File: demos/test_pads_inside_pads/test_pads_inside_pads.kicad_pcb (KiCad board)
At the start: 2 copper layers, 4 parts, among them P1 CONN_1, P2 CONN_1, P3 CONN_1, P4 CONN_1

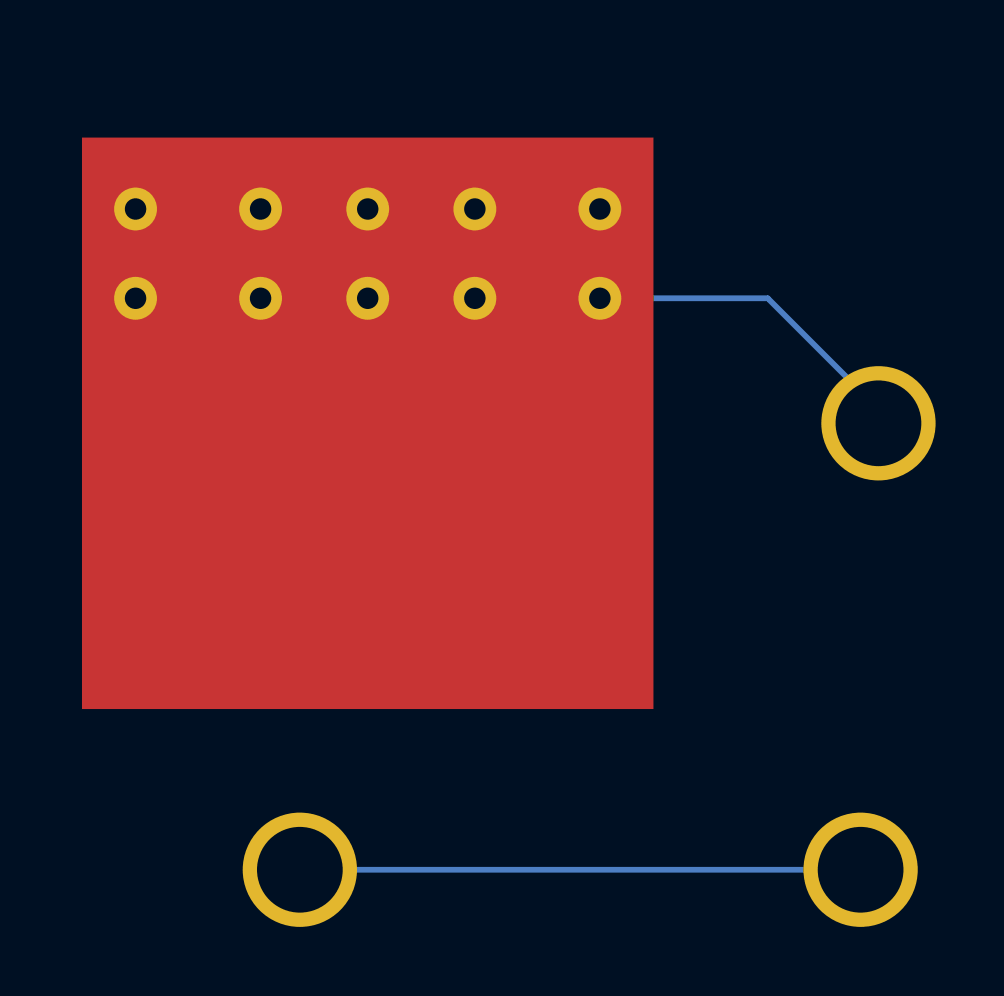
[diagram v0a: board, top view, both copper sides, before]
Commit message: Imported Upstream version 4.0.0~rc1
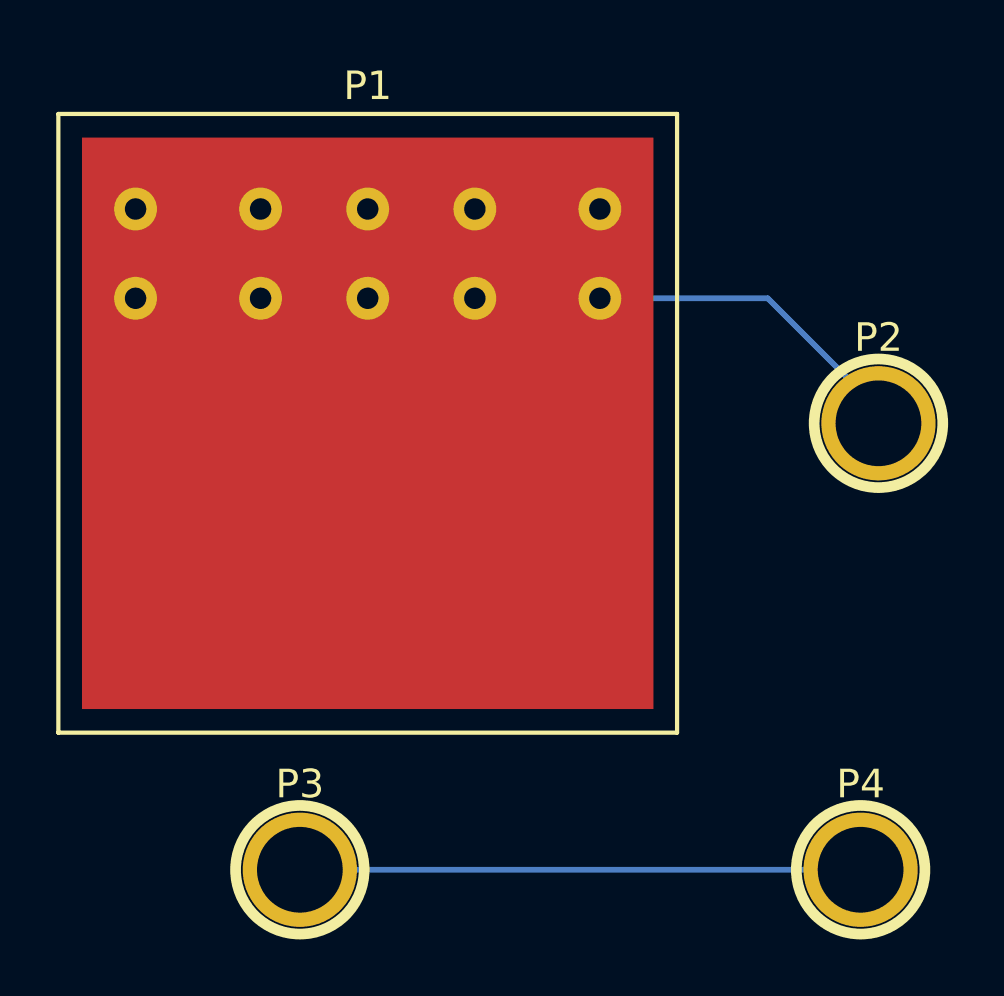
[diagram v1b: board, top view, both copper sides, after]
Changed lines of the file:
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@@
-(kicad_pcb (version 3) (host pcbnew "(2013-01-12 BZR 3902)-testing")
+(kicad_pcb (version 4) (host pcbnew "(2015-04-25 BZR 5623)-product")
   (general
     (links 12)
     (no_connects 0)
-    (area 74.91259 30.97059 111.463666 65.151)
+    (area 79.121 35.179 111.052429 65.3542)
     (thickness 1.6002)
     (drawings 0)
@@
   (page A4)
   (layers
-    (15 Dessus signal)
-    (0 Dessous signal)
-    (16 Dessous.Adhes user)
-    (17 Dessus.Adhes user)
-    (18 Dessous.Pate user)
-    (19 Dessus.Pate user)
-    (20 Dessous.SilkS user)
-    (21 Dessus.SilkS user)
-    (22 Dessous.Masque user)
-    (23 Dessus.Masque user)
-    (24 Dessin.User user)
-    (25 Cmts.User user)
-    (26 Eco1.User user)
-    (27 Eco2.User user)
-    (28 Contours.Ci user)
+    (0 Dessus signal)
+    (31 Dessous signal)
+    (32 B.Adhes user)
+    (33 F.Adhes user)
+    (34 B.Paste user)
+    (35 F.Paste user)
+    (36 B.SilkS user)
+    (37 F.SilkS user)
+    (38 B.Mask user)
+    (39 F.Mask user)
+    (40 Dwgs.User user)
+    (41 Cmts.User user)
+    (42 Eco1.User user)
+    (43 Eco2.User user)
+    (44 Edge.Cuts user)
   )
   (setup
@@
     (pad_to_mask_clearance 0.254)
     (aux_axis_origin 0 0)
-    (visible_elements FFFFFFBF)
+    (visible_elements 7FFFFFFF)
     (pcbplotparams
-      (layerselection 3178497)
+      (layerselection 0x00030_80000001)
       (usegerberextensions true)
       (excludeedgelayer true)
-      (linewidth 60)
+      (linewidth 0.150000)
       (plotframeref false)
       (viasonmask false)
@@
       (plotreference true)
       (plotvalue true)
-      (plotothertext true)
       (plotinvisibletext false)
       (padsonsilk false)
@@
     (uvia_dia 0.508)
     (uvia_drill 0.127)
-    (add_net "")
     (add_net /NET1)
     (add_net /NET2)
@@
     (descr "module 1 pin (ou trou mecanique de percage)")
     (tags DEV)
-    (fp_text reference P1 (at 0 -3.048) (layer Dessus.SilkS)
+    (fp_text reference P1 (at 0 -12) (layer F.SilkS)
       (effects (font (size 1.016 1.016) (thickness 0.254)))
     )
-    (fp_text value CONN_1 (at 0 2.794) (layer Dessus.SilkS) hide
+    (fp_text value CONN_1 (at 0 12) (layer F.SilkS) hide
       (effects (font (size 1.016 1.016) (thickness 0.254)))
     )
-    (fp_circle (center 0 0) (end 0 -2.286) (layer Dessus.SilkS) (width 0.381))
-    (pad 1 smd rect (at 0 0) (size 20.32 20.32)
-      (layers Dessus Dessus.Pate Dessus.Masque)
-      (net 2 /NET2)
-    )
-    (pad 1 thru_hole circle (at -8.255 -7.62) (size 1.524 1.524) (drill 0.762)
-      (layers *.Cu *.Mask Dessus.SilkS)
-      (net 2 /NET2)
-    )
-    (pad 1 thru_hole circle (at -3.81 -7.62) (size 1.524 1.524) (drill 0.762)
-      (layers *.Cu *.Mask Dessus.SilkS)
-      (net 2 /NET2)
-    )
-    (pad 1 thru_hole circle (at 0 -7.62) (size 1.524 1.524) (drill 0.762)
-      (layers *.Cu *.Mask Dessus.SilkS)
-      (net 2 /NET2)
-    )
-    (pad 1 thru_hole circle (at 3.81 -7.62) (size 1.524 1.524) (drill 0.762)
-      (layers *.Cu *.Mask Dessus.SilkS)
-      (net 2 /NET2)
-    )
-    (pad 1 thru_hole circle (at 8.255 -7.62) (size 1.524 1.524) (drill 0.762)
-      (layers *.Cu *.Mask Dessus.SilkS)
-      (net 2 /NET2)
-    )
-    (pad 1 thru_hole circle (at 8.255 -4.445) (size 1.524 1.524) (drill 0.762)
-      (layers *.Cu *.Mask Dessus.SilkS)
-      (net 2 /NET2)
-    )
-    (pad 1 thru_hole circle (at 3.81 -4.445) (size 1.524 1.524) (drill 0.762)
-      (layers *.Cu *.Mask Dessus.SilkS)
-      (net 2 /NET2)
-    )
-    (pad 1 thru_hole circle (at 0 -4.445) (size 1.524 1.524) (drill 0.762)
-      (layers *.Cu *.Mask Dessus.SilkS)
-      (net 2 /NET2)
-    )
-    (pad 1 thru_hole circle (at -3.81 -4.445) (size 1.524 1.524) (drill 0.762)
-      (layers *.Cu *.Mask Dessus.SilkS)
-      (net 2 /NET2)
-    )
-    (pad 1 thru_hole circle (at -8.255 -4.445) (size 1.524 1.524) (drill 0.762)
-      (layers *.Cu *.Mask Dessus.SilkS)
-      (net 2 /NET2)
-    )
+    (fp_line (start -11 -11) (end 11 -11) (layer F.SilkS) (width 0.15))
+    (fp_line (start 11 -11) (end 11 11) (layer F.SilkS) (width 0.15))
+    (fp_line (start 11 11) (end -11 11) (layer F.SilkS) (width 0.15))
+    (fp_line (start -11 11) (end -11 -11) (layer F.SilkS) (width 0.15))
+    (pad 1 smd rect (at 0 0) (size 20.32 20.32) (layers Dessus F.Paste F.Mask)
+      (net 2 /NET2))
+    (pad 1 thru_hole circle (at -8.255 -7.62) (size 1.524 1.524) (drill 0.762) (layers *.Cu *.Mask F.SilkS)
+      (net 2 /NET2))
+    (pad 1 thru_hole circle (at -3.81 -7.62) (size 1.524 1.524) (drill 0.762) (layers *.Cu *.Mask F.SilkS)
+      (net 2 /NET2))
+    (pad 1 thru_hole circle (at 0 -7.62) (size 1.524 1.524) (drill 0.762) (layers *.Cu *.Mask F.SilkS)
+      (net 2 /NET2))
+    (pad 1 thru_hole circle (at 3.81 -7.62) (size 1.524 1.524) (drill 0.762) (layers *.Cu *.Mask F.SilkS)
+      (net 2 /NET2))
+    (pad 1 thru_hole circle (at 8.255 -7.62) (size 1.524 1.524) (drill 0.762) (layers *.Cu *.Mask F.SilkS)
+      (net 2 /NET2))
+    (pad 1 thru_hole circle (at 8.255 -4.445) (size 1.524 1.524) (drill 0.762) (layers *.Cu *.Mask F.SilkS)
+      (net 2 /NET2))
+    (pad 1 thru_hole circle (at 3.81 -4.445) (size 1.524 1.524) (drill 0.762) (layers *.Cu *.Mask F.SilkS)
+      (net 2 /NET2))
+    (pad 1 thru_hole circle (at 0 -4.445) (size 1.524 1.524) (drill 0.762) (layers *.Cu *.Mask F.SilkS)
+      (net 2 /NET2))
+    (pad 1 thru_hole circle (at -3.81 -4.445) (size 1.524 1.524) (drill 0.762) (layers *.Cu *.Mask F.SilkS)
+      (net 2 /NET2))
+    (pad 1 thru_hole circle (at -8.255 -4.445) (size 1.524 1.524) (drill 0.762) (layers *.Cu *.Mask F.SilkS)
+      (net 2 /NET2))
   )
   (module 1pin (layer Dessus)
@@
     (descr "module 1 pin (ou trou mecanique de percage)")
     (tags DEV)
-    (fp_text reference P2 (at 0 -3.048) (layer Dessus.SilkS)
+    (fp_text reference P2 (at 0 -3.048) (layer F.SilkS)
       (effects (font (size 1.016 1.016) (thickness 0.254)))
     )
-    (fp_text value CONN_1 (at 0 2.794) (layer Dessus.SilkS) hide
+    (fp_text value CONN_1 (at 0 2.794) (layer F.SilkS) hide
       (effects (font (size 1.016 1.016) (thickness 0.254)))
     )
-    (fp_circle (center 0 0) (end 0 -2.286) (layer Dessus.SilkS) (width 0.381))
-    (pad 1 thru_hole circle (at 0 0) (size 4.064 4.064) (drill 3.048)
-      (layers *.Cu *.Mask Dessus.SilkS)
-      (net 2 /NET2)
-    )
+    (fp_circle (center 0 0) (end 0 -2.286) (layer F.SilkS) (width 0.381))
+    (pad 1 thru_hole circle (at 0 0) (size 4.064 4.064) (drill 3.048) (layers *.Cu *.Mask F.SilkS)
+      (net 2 /NET2))
   )
   (module 1pin (layer Dessus)
@@
     (descr "module 1 pin (ou trou mecanique de percage)")
     (tags DEV)
-    (fp_text reference P3 (at 0 -3.048) (layer Dessus.SilkS)
+    (fp_text reference P3 (at 0 -3.048) (layer F.SilkS)
       (effects (font (size 1.016 1.016) (thickness 0.254)))
     )
-    (fp_text value CONN_1 (at 0 2.794) (layer Dessus.SilkS) hide
+    (fp_text value CONN_1 (at 0 2.794) (layer F.SilkS) hide
       (effects (font (size 1.016 1.016) (thickness 0.254)))
     )
-    (fp_circle (center 0 0) (end 0 -2.286) (layer Dessus.SilkS) (width 0.381))
-    (pad 1 thru_hole circle (at 0 0) (size 4.064 4.064) (drill 3.048)
-      (layers *.Cu *.Mask Dessus.SilkS)
-      (net 1 /NET1)
-    )
+    (fp_circle (center 0 0) (end 0 -2.286) (layer F.SilkS) (width 0.381))
+    (pad 1 thru_hole circle (at 0 0) (size 4.064 4.064) (drill 3.048) (layers *.Cu *.Mask F.SilkS)
+      (net 1 /NET1))
   )
   (module 1pin (layer Dessus)
@@
     (descr "module 1 pin (ou trou mecanique de percage)")
     (tags DEV)
-    (fp_text reference P4 (at 0 -3.048) (layer Dessus.SilkS)
+    (fp_text reference P4 (at 0 -3.048) (layer F.SilkS)
       (effects (font (size 1.016 1.016) (thickness 0.254)))
     )
-    (fp_text value CONN_1 (at 0 2.794) (layer Dessus.SilkS) hide
+    (fp_text value CONN_1 (at 0 2.794) (layer F.SilkS) hide
       (effects (font (size 1.016 1.016) (thickness 0.254)))
     )
-    (fp_circle (center 0 0) (end 0 -2.286) (layer Dessus.SilkS) (width 0.381))
-    (pad 1 thru_hole circle (at 0 0) (size 4.064 4.064) (drill 3.048)
-      (layers *.Cu *.Mask Dessus.SilkS)
-      (net 1 /NET1)
-      (die_length 7.62)
-    )
+    (fp_circle (center 0 0) (end 0 -2.286) (layer F.SilkS) (width 0.381))
+    (pad 1 thru_hole circle (at 0 0) (size 4.064 4.064) (drill 3.048) (layers *.Cu *.Mask F.SilkS)
+      (net 1 /NET1) (die_length 7.62))
   )
   (segment (start 107.061 61.468) (end 87.122 61.468) (width 0.2032) (layer Dessous) (net 1))
+  (segment (start 103.759 41.148) (end 107.696 45.085) (width 0.2032) (layer Dessous) (net 2))
+  (segment (start 107.696 45.085) (end 107.696 45.593) (width 0.2032) (layer Dessous) (net 2))
   (segment (start 97.79 41.148) (end 103.759 41.148) (width 0.2032) (layer Dessous) (net 2))
-  (segment (start 107.696 45.085) (end 107.696 45.593) (width 0.2032) (layer Dessous) (net 2))
-  (segment (start 103.759 41.148) (end 107.696 45.085) (width 0.2032) (layer Dessous) (net 2))
 )
